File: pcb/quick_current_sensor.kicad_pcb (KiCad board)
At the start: 2 copper layers, 66.2 x 51.8 mm, 22 parts, among them J3 +LOAD, J4 -LOAD, Q1 MTP2P50E, U1 LM358N, U2 TL431LP

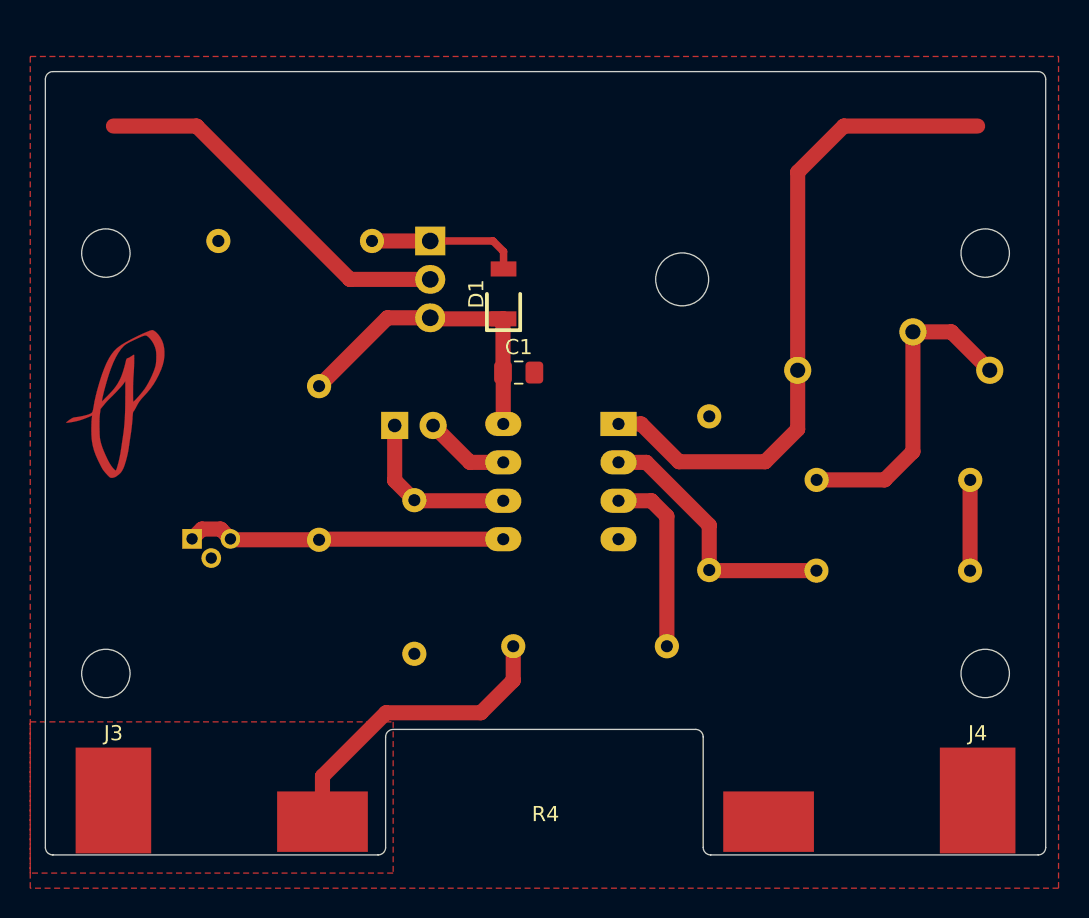
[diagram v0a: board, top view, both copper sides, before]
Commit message: cleanup, reduce size
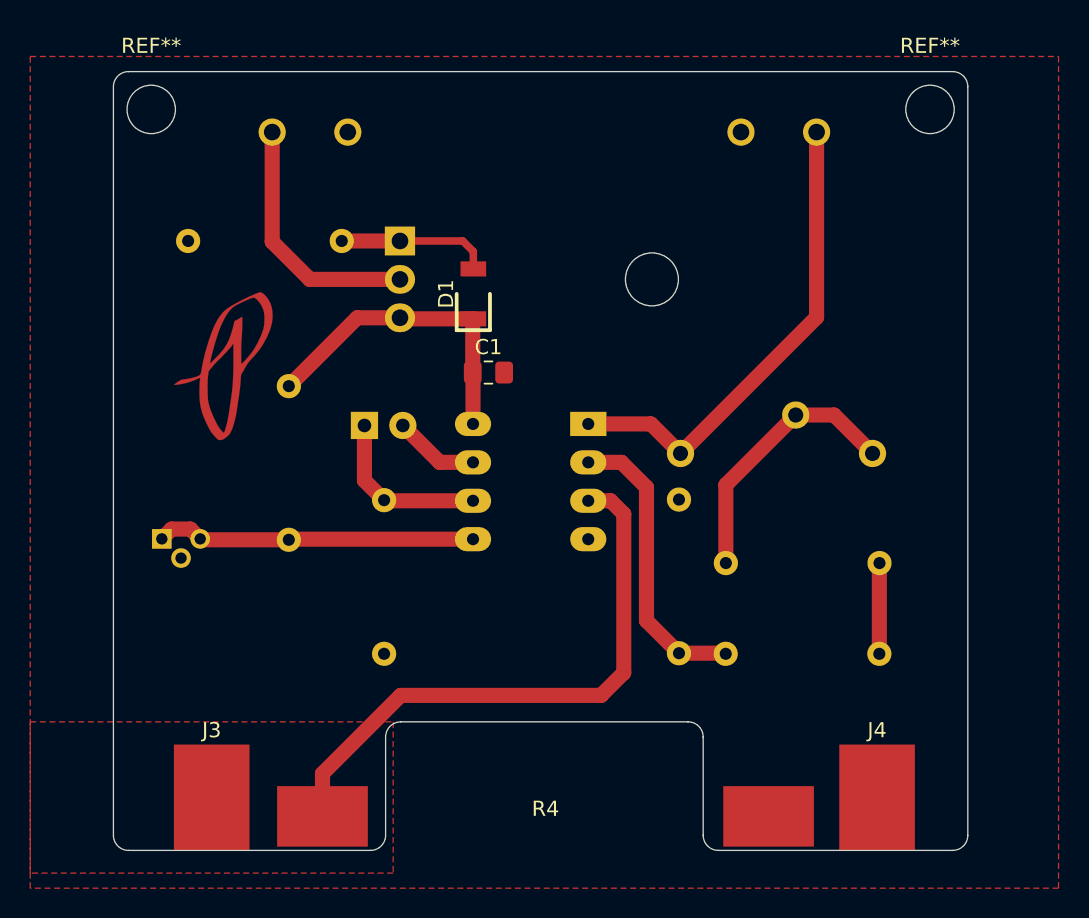
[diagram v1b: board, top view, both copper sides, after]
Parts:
- removed H1, H2, H3, H4: MountingHole, MountingHole:MountingHole_3.2mm_M3
- removed R8: 0, Resistor_THT:R_Axial_DIN0207_L6.3mm_D2.5mm_P10.16mm_Horizontal
- added J1: PWR, pl_TerminalBlock:WJ127-5.0-2P, B.Cu at (95.0, 74.0)
- added J2: OUT, pl_TerminalBlock:WJ127-5.0-2P, B.Cu at (131.0, 74.0)
- added REF**: MountingHole_3.2mm_M3, MountingHole:MountingHole_3.2mm_M3, F.Cu at (138.5, 72.5)
- added REF**: MountingHole_3.2mm_M3, MountingHole:MountingHole_3.2mm_M3, F.Cu at (87.0, 72.5)
- J4: value -LOAD -> GND
- moved RV1 9.50 mm to (122.0, 95.2)
- moved R2 8.14 mm to (135.2, 108.5)
- moved R3 8.14 mm to (125.0, 102.5)
- moved G*** 7.57 mm to (91.8, 89.5)
- moved J4 6.65 mm to (135.0, 118.0)
- moved J3 6.50 mm to (91.0, 118.0)
- moved R1 5.85 mm to (121.9, 98.3)
- moved C1 2.00 mm to (109.3, 89.9)
- moved D1 2.00 mm to (108.3, 84.7)
- moved D2 2.00 mm to (101.1, 93.4)
- moved Q1 2.00 mm to (103.5, 81.2)
- moved R5 2.00 mm to (99.6, 81.2)
- moved R6 2.00 mm to (96.1, 90.8)
- moved R7 2.00 mm to (102.4, 108.5)
- moved U1 2.00 mm to (115.9, 93.3)
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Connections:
- U1 pad 3: Net-(R8-Pad1) -> Net-(J3-Pad1)
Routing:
- net Net-(J3-Pad1): track 20.5 -> 38.7 mm
- net Net-(R8-Pad1): track 12.2 -> 0.00 mm
- net Net-(J2-Pad1): track 43.9 -> 31.9 mm
- net Net-(J1-Pad1): track 25.2 -> 16.7 mm
- net Net-(R3-Pad1): track 21.2 -> 17.8 mm
- net Net-(R1-Pad2): track 17.8 -> 19.5 mm
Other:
- board size 66.2 x 51.8 mm -> 56.5 x 51.5 mm
